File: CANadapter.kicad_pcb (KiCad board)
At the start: 2 copper layers, 47 x 22.9 mm, 27 parts, among them P1 CONN_02X06, P2 CONN_01X06, P3 CONN_01X04, U1 MCP2515, U2 TLP2361, U3 TLP2361, U4 MCP2551-I/SN, U5 LM7805CT, Y1 16MHz

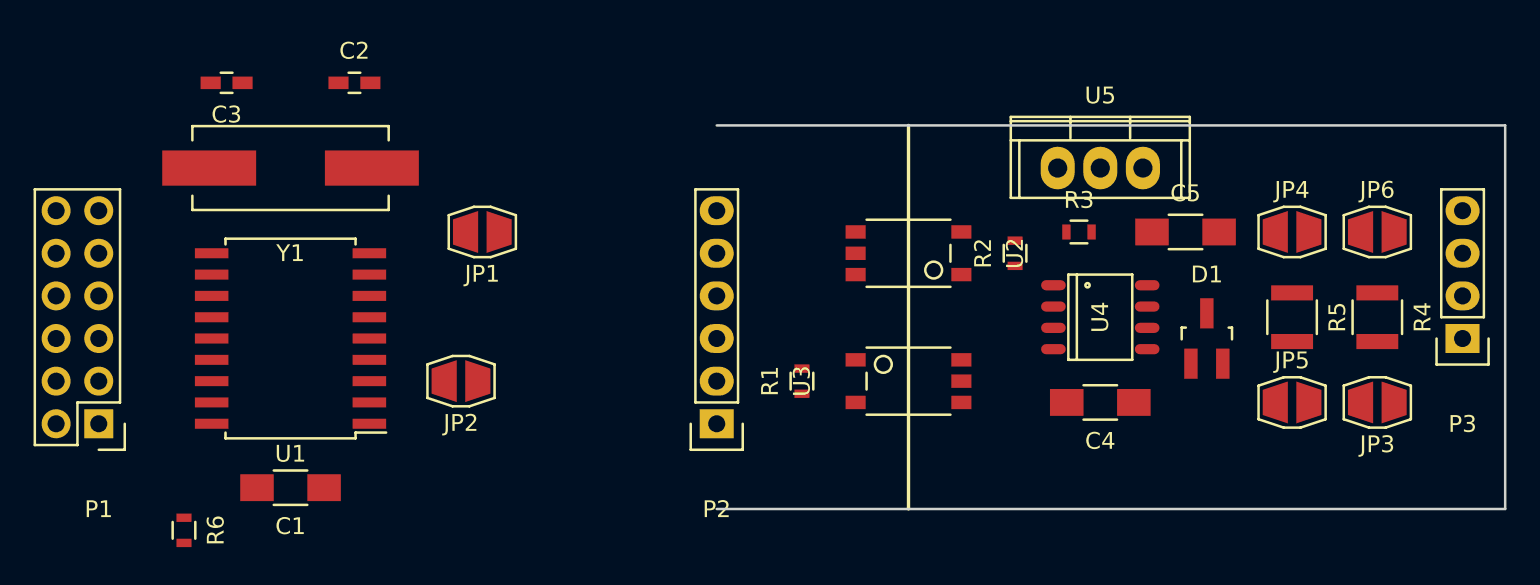
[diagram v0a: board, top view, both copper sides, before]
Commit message: Partial layout
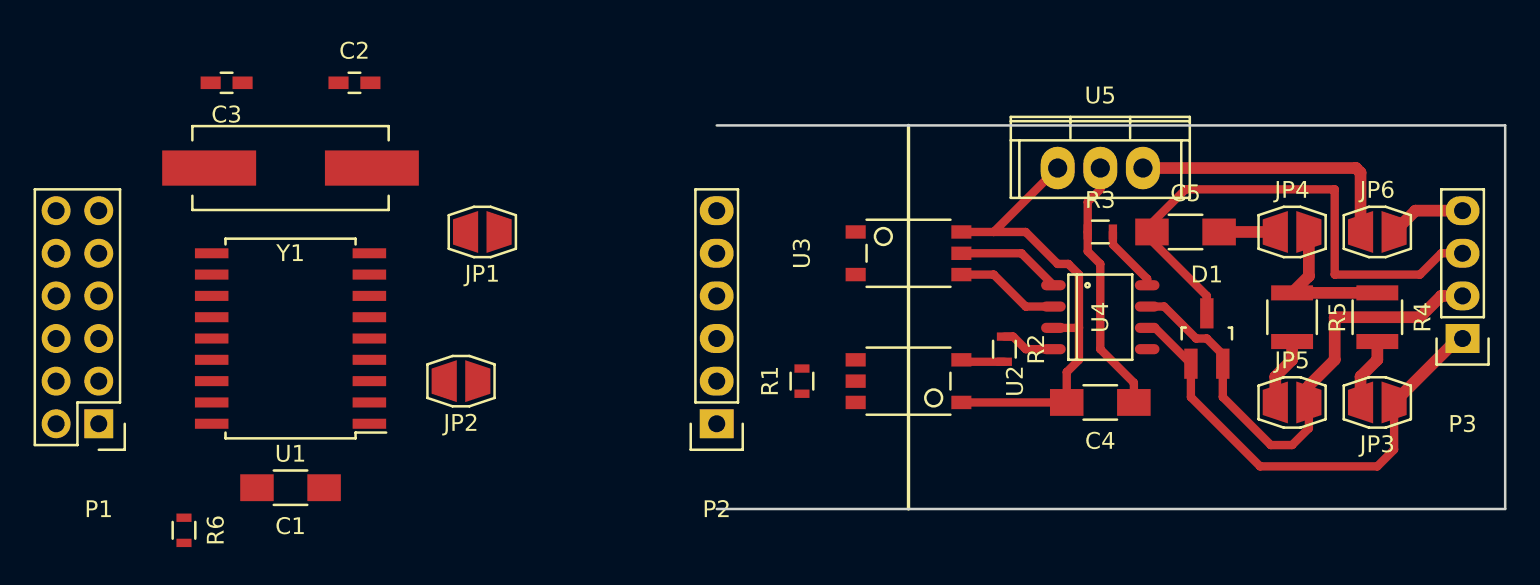
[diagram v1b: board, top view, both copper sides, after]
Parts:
- moved U2 7.62 mm to (144.8, 109.2)
- moved U3 7.62 mm to (144.8, 101.6)
- moved R2 5.75 mm to (150.5, 107.3), turned to 270 degrees
- moved R3 1.27 mm to (156.2, 100.3)
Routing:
- net GNDREF: track 0.00 -> 53.9 mm
- net /CAN_H: track 0.00 -> 30.4 mm
- net +5V: track 0.00 -> 29.7 mm
- net /CAN_L: track 0.00 -> 28.2 mm
- net Net-(JP6-Pad2): track 0.00 -> 16.6 mm
- net Net-(JP4-Pad1): track 0.00 -> 9.12 mm
- net Net-(U3-Pad5): track 0.00 -> 6.28 mm
- net +12V: track 0.00 -> 4.61 mm
- net Net-(R3-Pad2): track 0.00 -> 4.28 mm
- net Net-(JP5-Pad2): track 0.00 -> 4.04 mm
- net Net-(JP3-Pad1): track 0.00 -> 4.04 mm
- net Net-(C5-Pad2): track 0.00 -> 3.35 mm
- net Net-(R2-Pad1): track 0.00 -> 3.23 mm
- net Net-(R2-Pad2): track 0.00 -> 2.61 mm
